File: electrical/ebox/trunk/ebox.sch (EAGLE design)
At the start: 161 parts, among them IC1 MAX3221CUE, IC10 SN74LVC1G125, IC11 MAX3221CUE, IC12 INA170, IC13 SN74LVC1G125, IC14 SN74LVC1G125, IC15 MAX3221CUE, IC16 MCP170333MB, IC17 SN74LVC1G125, IC18 SN74LVC1G125, IC19 74ALS04D, IC2 LT3652, IC3 XMEGA128A1, IC4 LT1161, IC5 SN74LVC1G125, IC6 SN74LVC1G125, IC7 MAX3221CUE, IC8 INA170, IC9 SN74LVC1G125, Q1 FDD4141TO252, U1 BLUETOOTH-RN42, U2 D2523T_, X1 7381-3PG-300, X10 DEANS-MALE, X11 B4B-ZR, X12 DEANS-MALE, X13 B4B-ZR, X14 22-23-2021, X15 DEANS-FEMALE, X16 DEANS-FEMALE, X17 USB_A, X18 22-23-2021, X2 7381-3PG-300, X3 7381-2PG-300, X4 17984-7PG-300, X5 17984-7PG-300, X6 17984-7PG-300, X7 17984-7PG-300, X8 22-23-2031, X9 22-23-2031

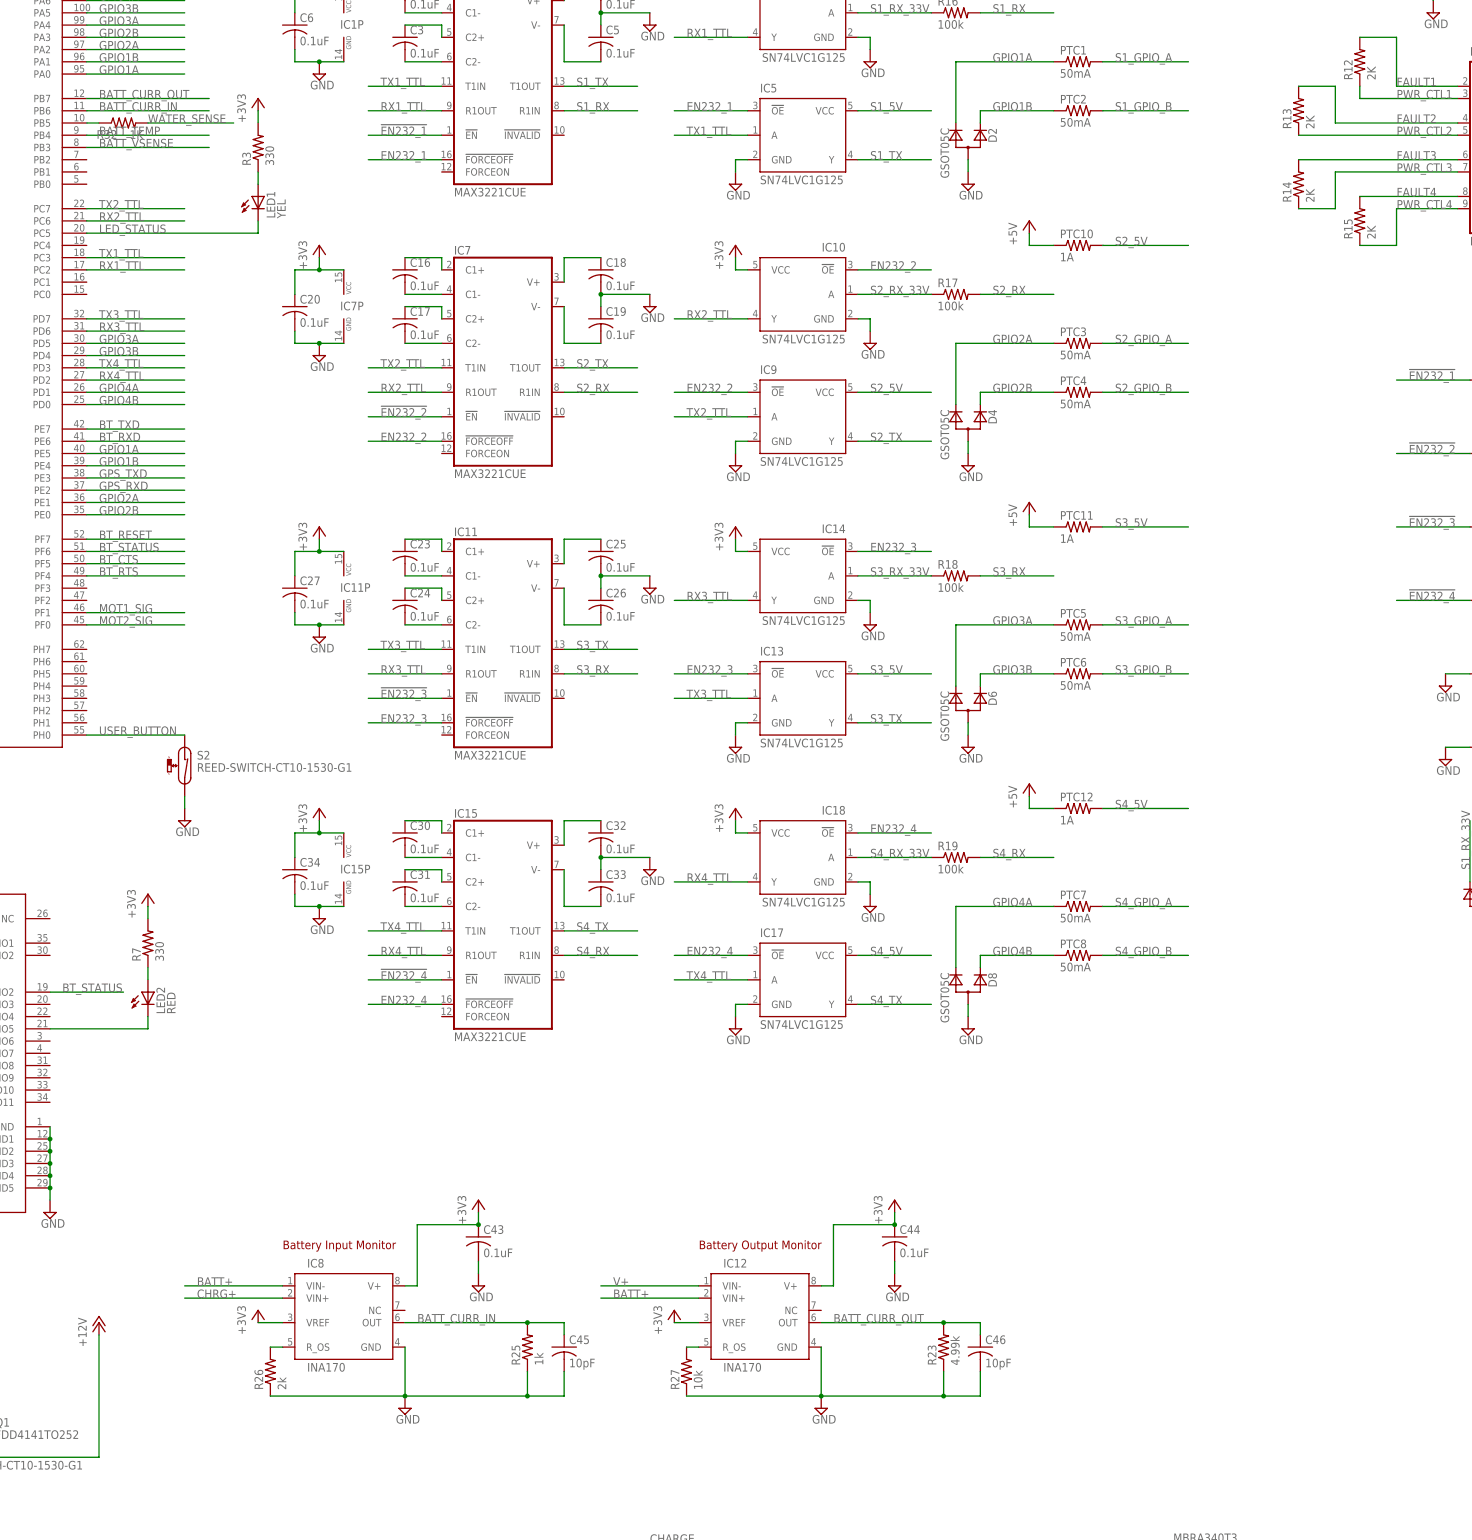
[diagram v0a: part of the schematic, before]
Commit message: Cleaned up more stuff.  Just need to do final check and silkscreen work.
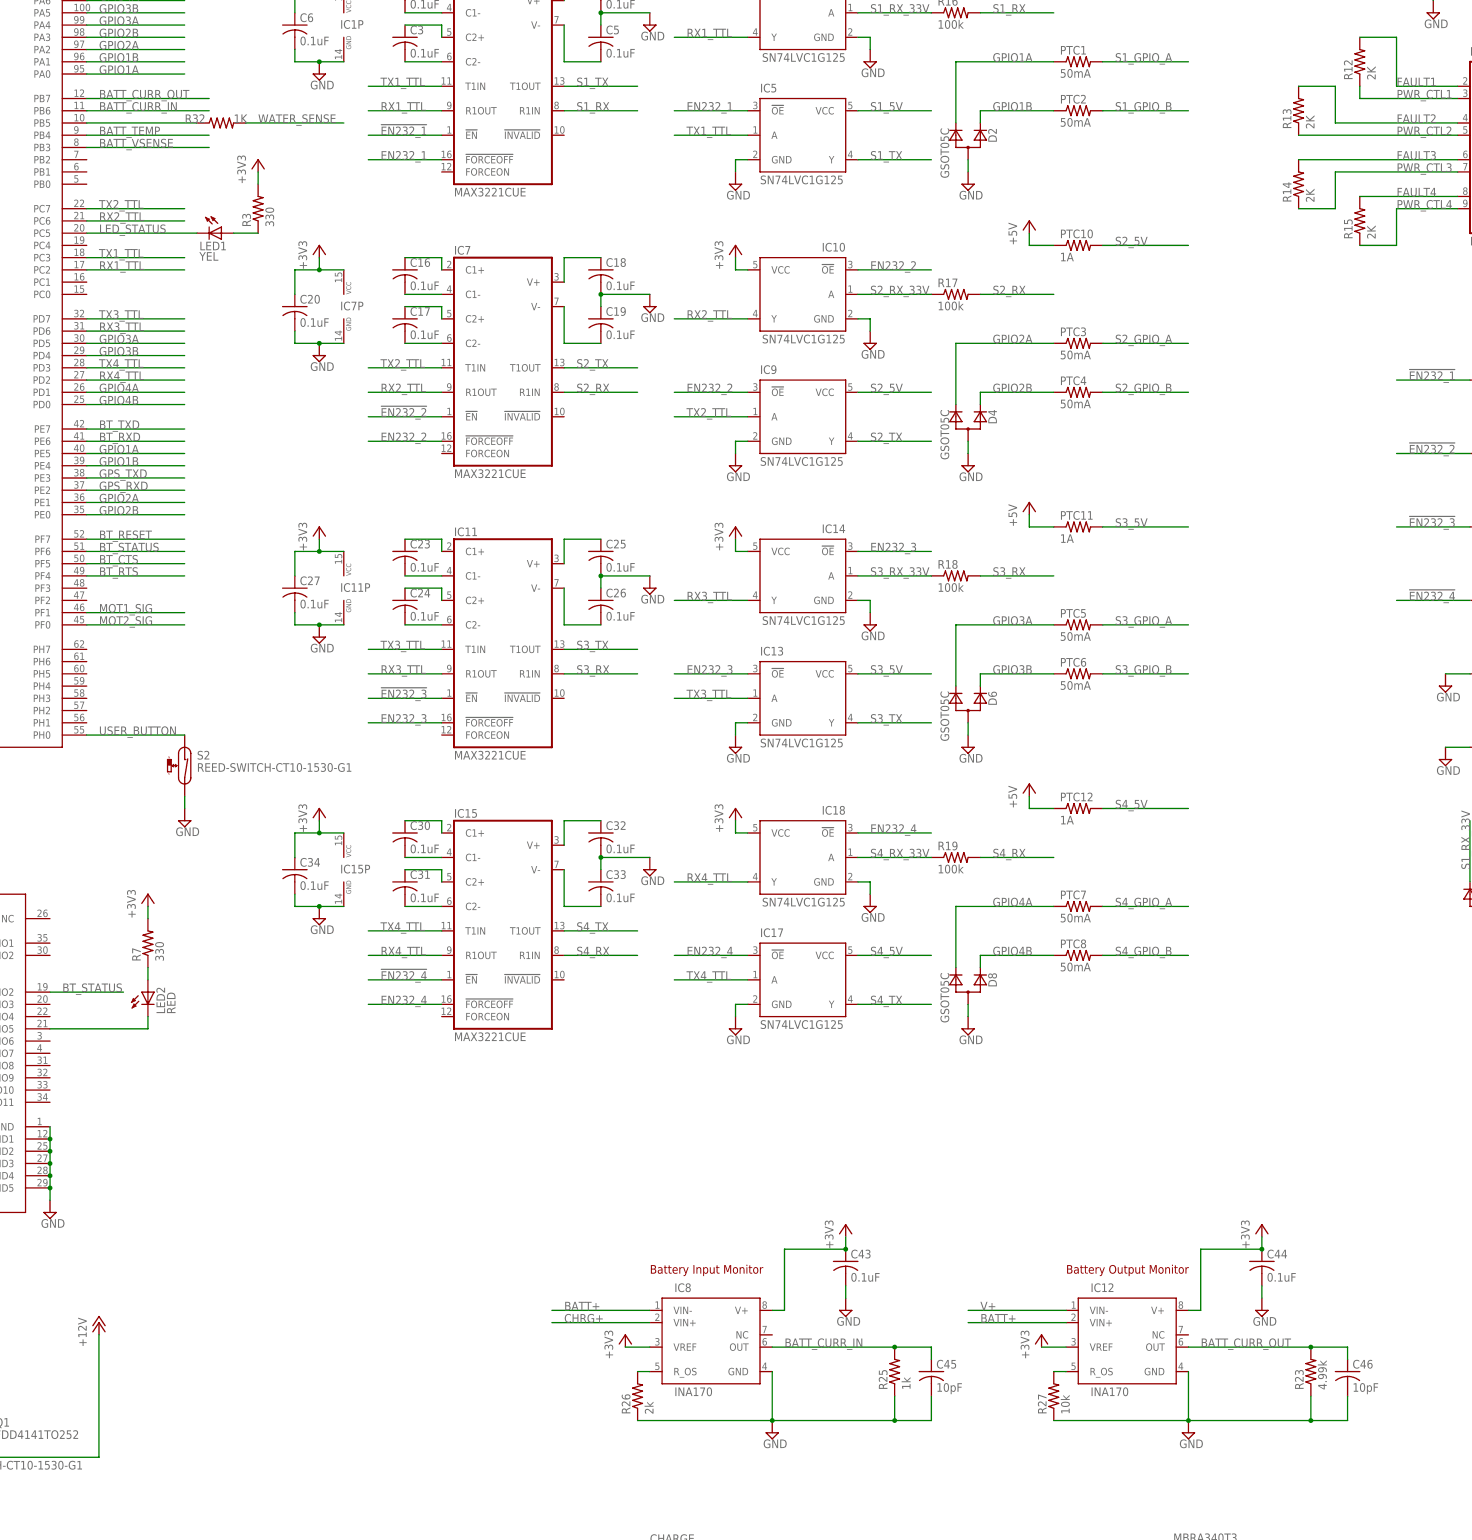
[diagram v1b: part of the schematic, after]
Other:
- moved on the sheet: C43, C44, C45, C46, IC12, IC8, LED1, R23, R25, R26, R27, R3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
